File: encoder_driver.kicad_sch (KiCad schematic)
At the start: 16 parts, among them J1 Conn_01x10_Female, J2 Conn_01x02_Male, J2 Conn_01x10_Female, J3 Conn_01x07, Q1 Si2319CDS, U1 AS5045B, U2 AM26LS31CD, U3 AM26LV32xD

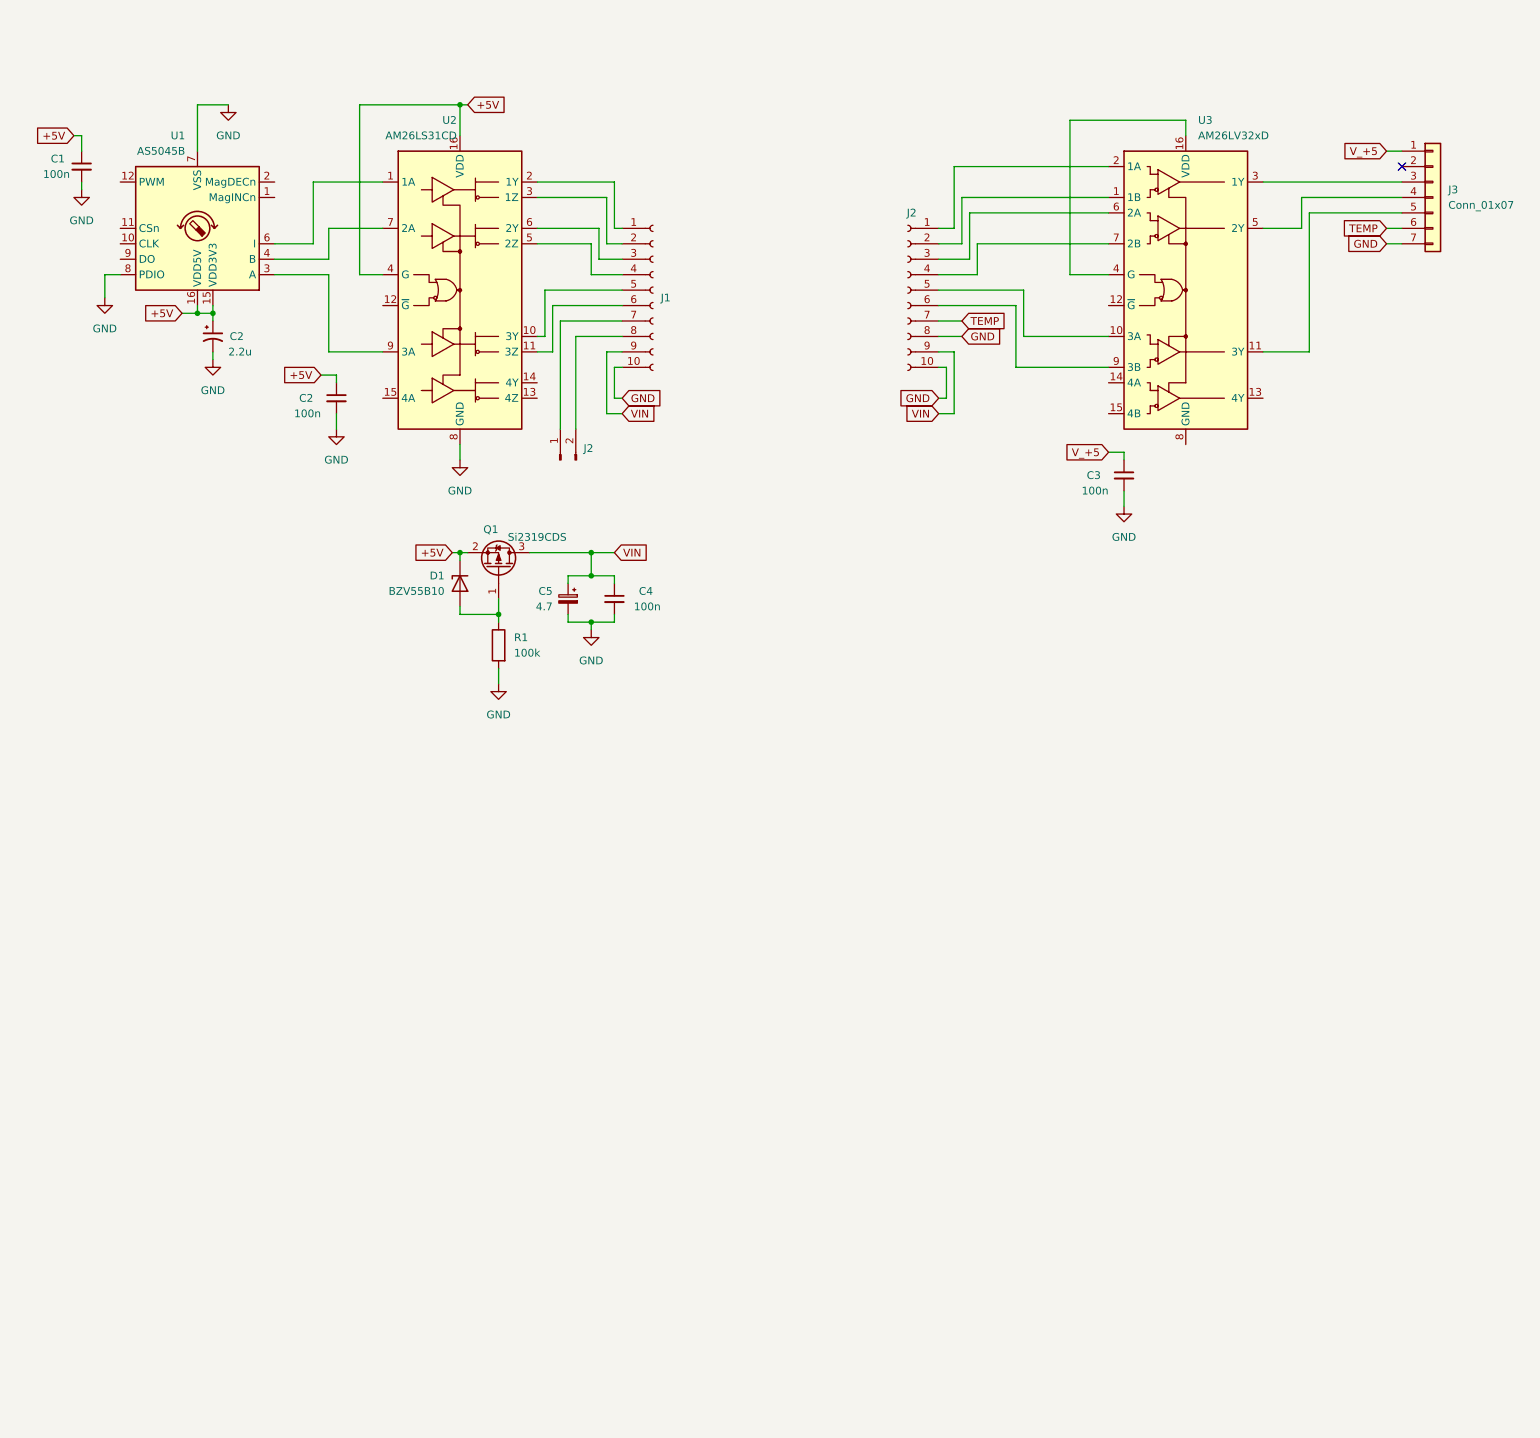
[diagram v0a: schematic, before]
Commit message: finished draft schematic
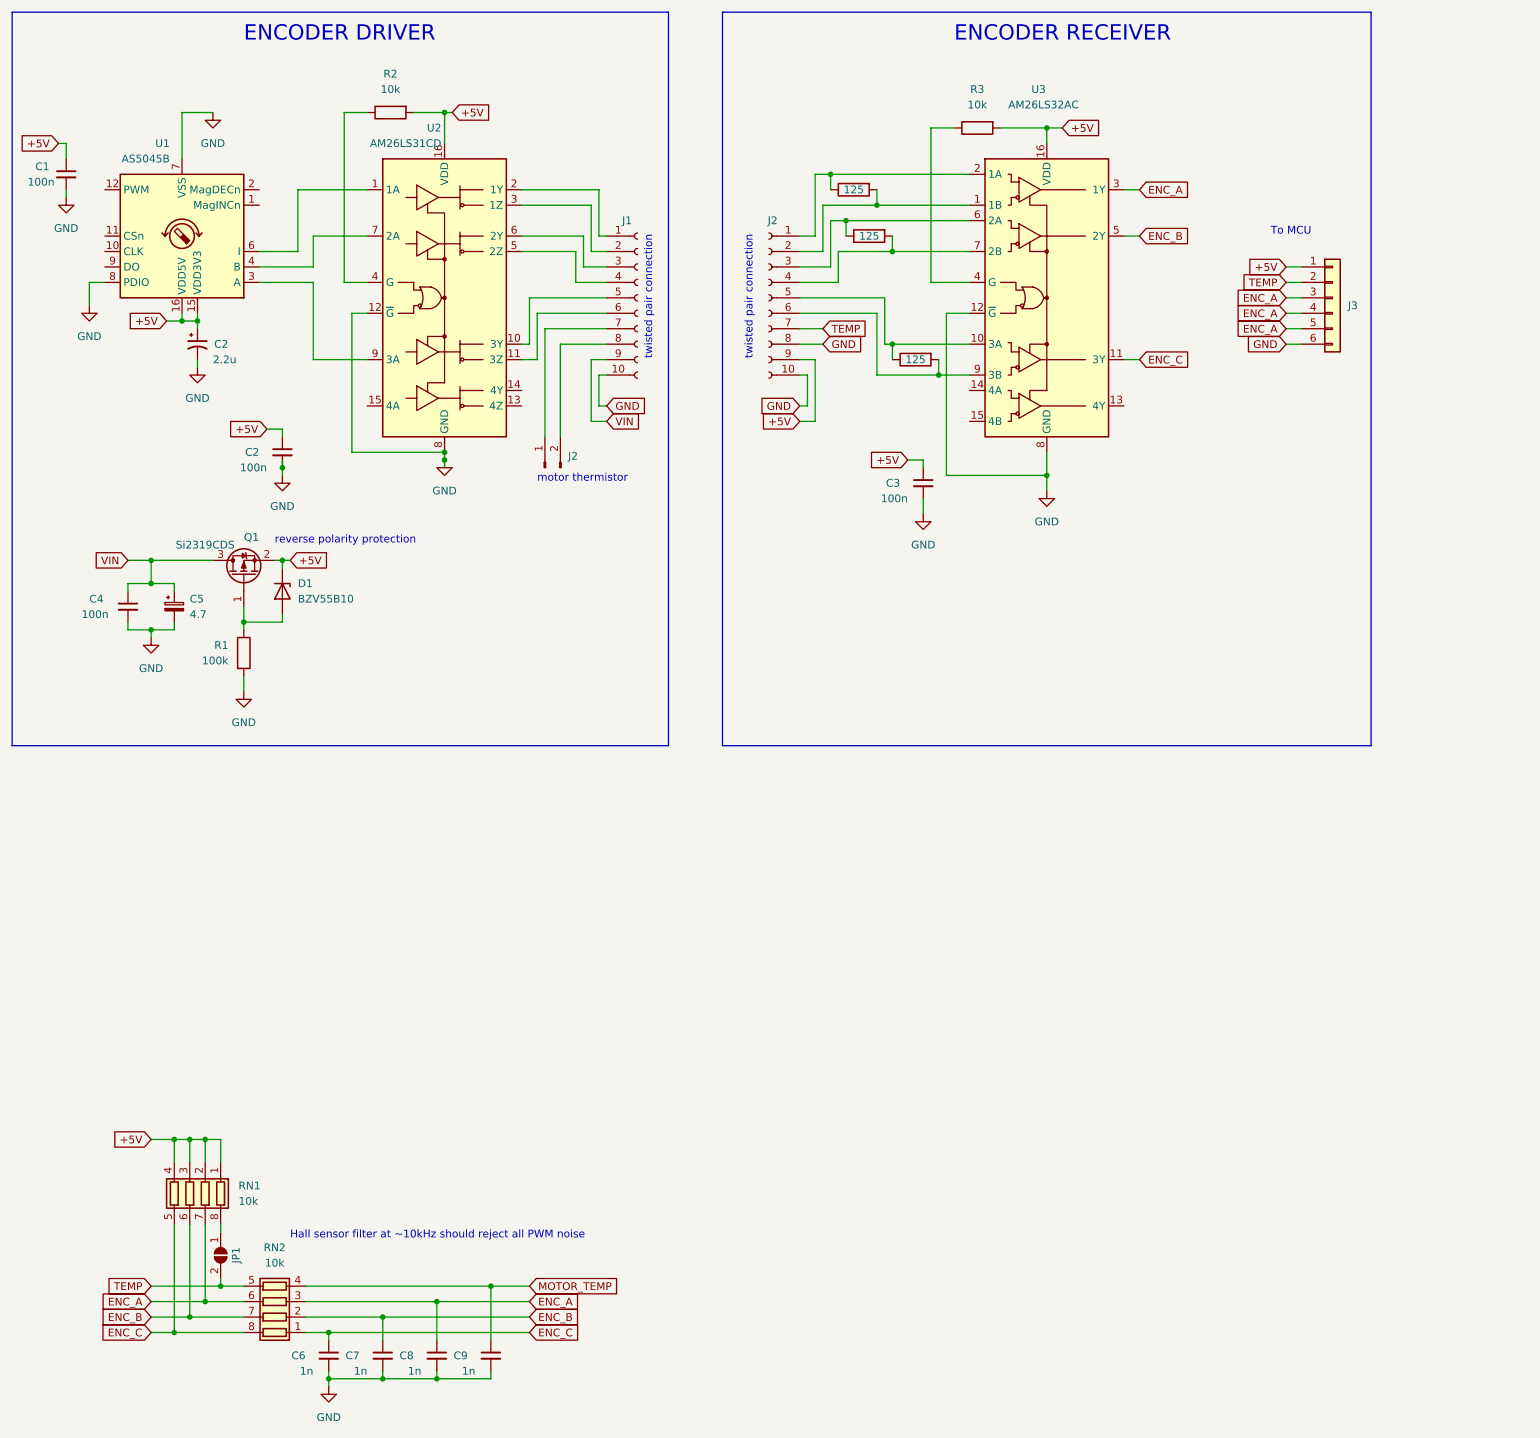
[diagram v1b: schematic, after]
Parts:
- added C6, C7, C8, C9: 1n, symbol Device:C_Small
- added JP1: SolderJumper_2_Open, symbol Jumper:SolderJumper_2_Open
- added R2, R3: 10k, symbol Device:R
- added R? (x3): 125, symbol Device:R
- added RN1, RN2: 10k, Resistor_SMD:R_Array_Concave_4x0603, symbol Device:R_Pack04
- J3: symbol Connector_Generic:Conn_01x07 -> Connector_Generic:Conn_01x06
- U3: value AM26LV32xD -> AM26LS32AC
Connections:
- net V_+5 is gone; now on net +5V: C3.1, J3.1 (Pin_1)
- net +5V: now also J2.9 (Pin_9), U3.16 (VDD), R2.2, R3.2, RN1.1 (R1.1), RN1.2 (R2.1), RN1.3 (R3.1), RN1.4 (R4.1); no longer U2.4 (G)
- net GND: now also J3.6 (Pin_6), U2.12 (~{G}), U3.12 (~{G}), U3.8 (GND), C6.2, C7.2, C8.2, C9.2; no longer J3.7 (Pin_7)
- net TEMP: now also J3.2 (Pin_2), JP1.2 (B), RN2.5 (R4.2); no longer J3.6 (Pin_6)
- net VIN: no longer J2.9 (Pin_9)
- net at J2.2 (Pin_2), U3.1 (1B): now also R?.2
- net at J2.5 (Pin_5), U3.10 (3A): now also R?.1
- net ENC_A: now reaches J3.5 (Pin_5)
- net ENC_A: now also J3.3 (Pin_3), J3.4 (Pin_4), U3.3 (1Y), C8.1, RN1.7 (R2.2), RN2.3 (R3.1), RN2.6 (R3.2); no longer U3.11 (3Y)
- net at U3.4 (G): now also R3.1; no longer U3.16 (VDD)
- net at J2.1 (Pin_1), U3.2 (1A): now also R?.1
- net ENC_B: now reaches U3.5 (2Y)
- net ENC_B: now also C7.1, RN1.6 (R3.2), RN2.2 (R2.1), RN2.7 (R2.2); no longer J3.4 (Pin_4)
- net at J2.3 (Pin_3), U3.6 (2A): now also R?.1
- net at J2.4 (Pin_4), U3.7 (2B): now also R?.2
- net at J2.6 (Pin_6), U3.9 (3B): now also R?.2
- new net: R2.1, U2.4 (G)
- new net: JP1.1 (A), RN1.8 (R1.2)
- new net ENC_C: C6.1, RN1.5 (R4.2), RN2.1 (R1.1), RN2.8 (R1.2), U3.11 (3Y)
- new net MOTOR_TEMP: C9.1, RN2.4 (R4.1)
- no-connect marks 1 -> 0
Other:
- note added: "ENCODER DRIVER"
- note added: "ENCODER RECEIVER"
- note added: "Hall sensor filter at ~10kHz should reject all PWM noise"
- note added: "To MCU"
- note added: "motor thermistor"
- note added: "reverse polarity protection"
- note added: "twisted pair connection"
- moved on the sheet: C1, C2, C3, C4, C5, D1, J1, J2, Q1, R1, U1, U2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
